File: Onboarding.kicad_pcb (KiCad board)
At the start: 2 copper layers, 45.7 x 45.7 mm, 20 parts, among them J1 Conn_01x02, J2 Conn_01x02, J3 Conn_01x02, J4 Conn_01x02, U2 MC34063A

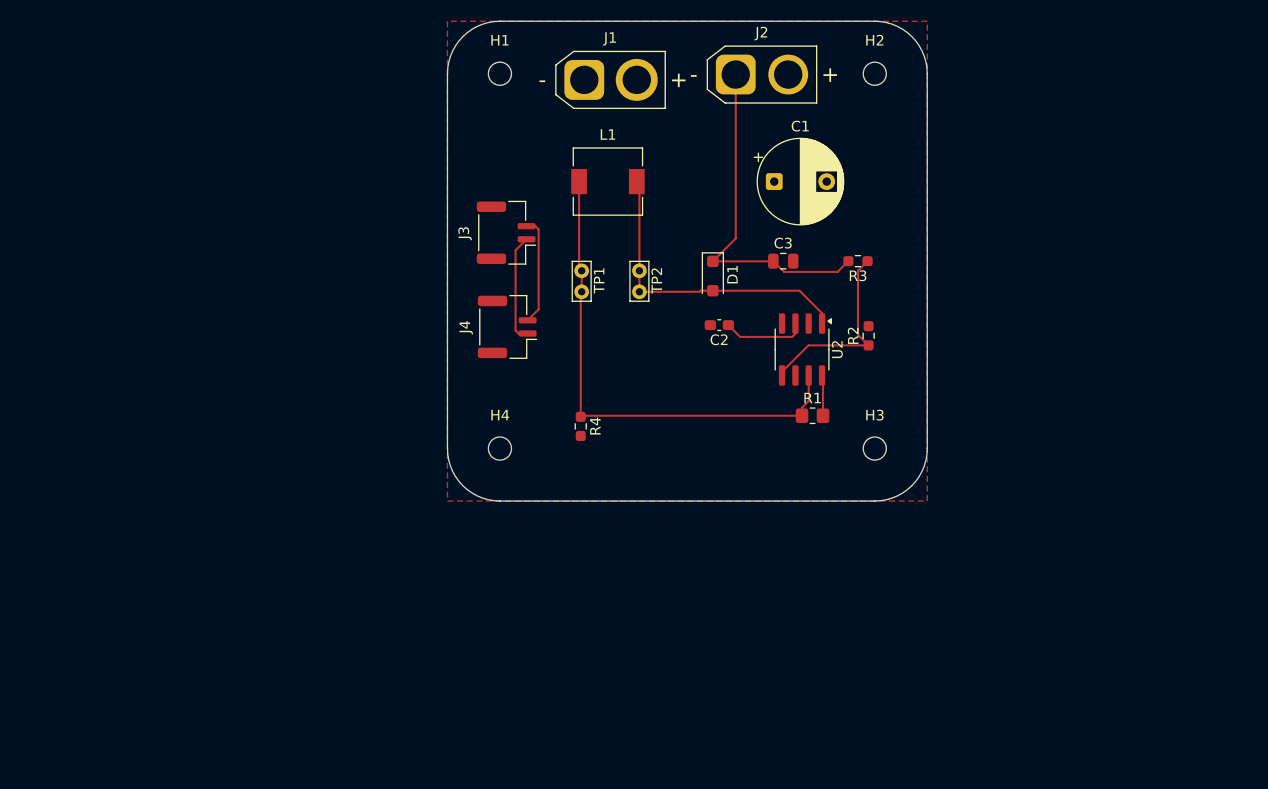
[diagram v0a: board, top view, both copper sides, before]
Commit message: Update PCB
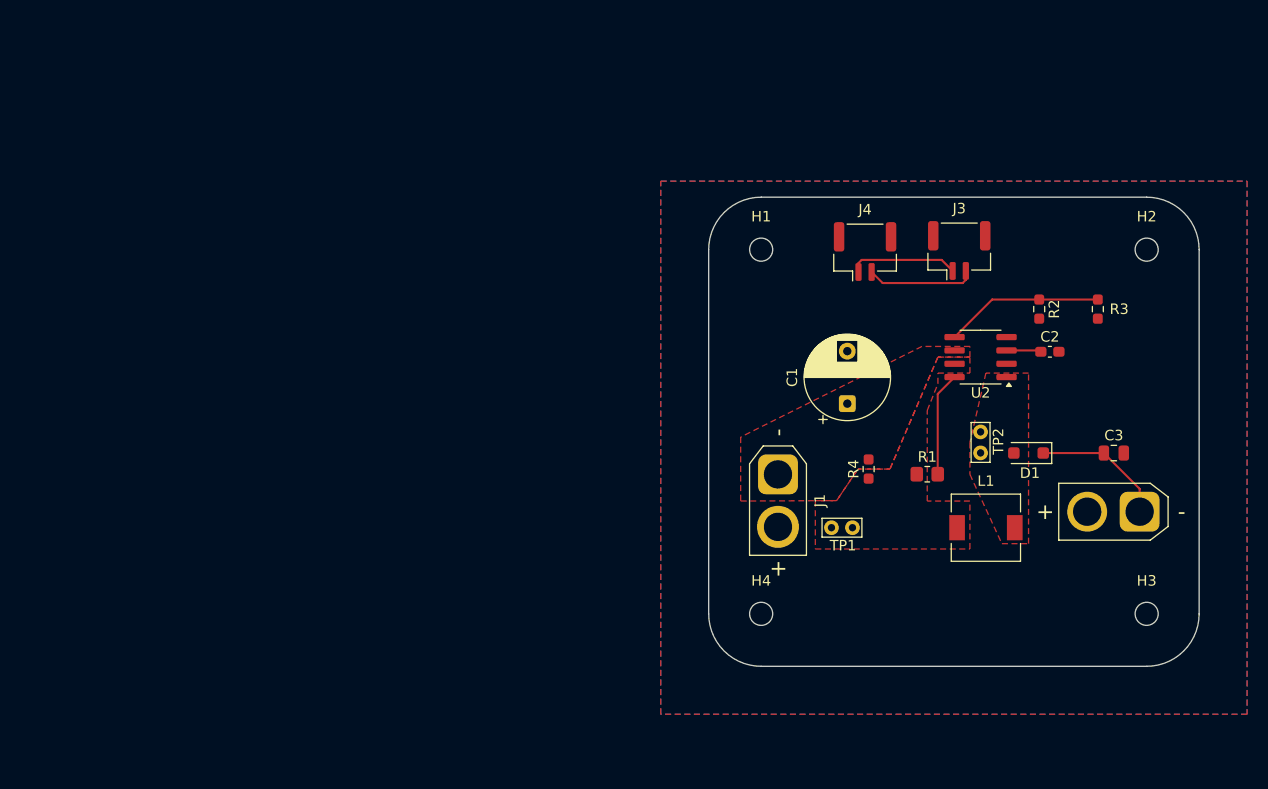
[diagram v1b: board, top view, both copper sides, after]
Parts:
- moved J2 56.7 mm to (253.9, 92.5), turned to 180 degrees
- moved L1 48.8 mm to (239.3, 94.0)
- moved J3 43.2 mm to (236.7, 67.6), turned to 0 degrees
- moved J1 41.9 mm to (219.5, 88.9), turned to -90 degrees
- moved C3 36.4 mm to (251.5, 86.9)
- moved TP2 36.0 mm to (238.8, 86.9)
- moved J4 34.9 mm to (227.8, 67.7), turned to 0 degrees
- moved D1 34.5 mm to (243.3, 86.9), turned to 180 degrees
- moved TP1 32.7 mm to (224.6, 94.0), turned to 0 degrees
- moved C2 31.6 mm to (245.4, 77.2), turned to 0 degrees
- moved H2 30.9 mm to (254.6, 67.5)
- moved H3 30.3 mm to (254.6, 102.2)
- moved H1 30.0 mm to (217.9, 67.5)
- moved H4 29.5 mm to (217.9, 102.2)
- moved R4 27.7 mm to (228.1, 88.4), turned to 90 degrees
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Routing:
- net Net-(U2-I_{PK}): track 47.8 -> 0.00 mm
- net Net-(D1-A): track 29.9 -> 0.00 mm
- net VCC: track 32.5 -> 12.8 mm
- net Net-(U2-DC): track 3.88 -> 9.92 mm
- net Net-(U2-CT): track 7.95 -> 3.32 mm
- net Net-(U2-COMP-): track 18.5 -> 15.1 mm
- added copper zone on B.Cu, net GND
- added copper zone on F.Cu, net GND
- added copper zone on F.Cu, net Net-(D1-A)
- added copper zone on F.Cu, net Net-(U2-I_{PK})
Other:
- board size 45.7 x 45.7 mm -> 46.7 x 44.7 mm

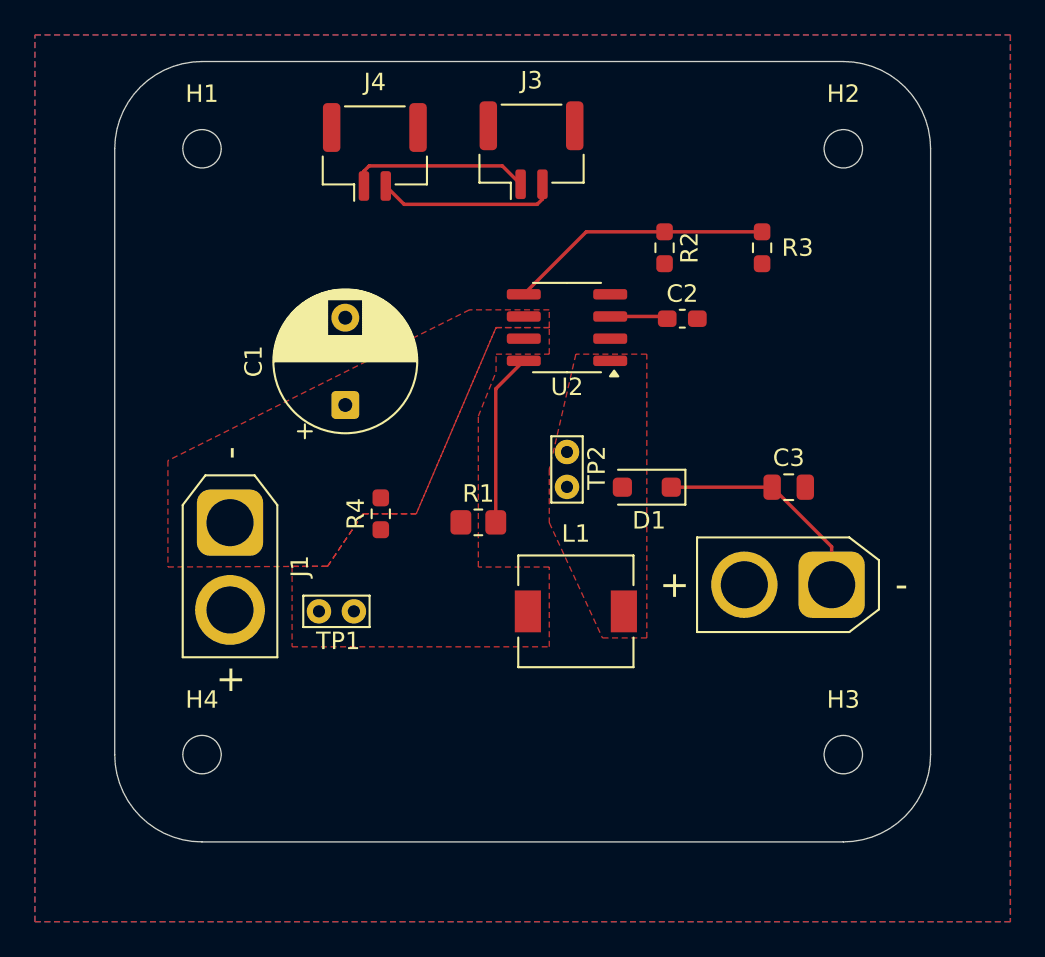
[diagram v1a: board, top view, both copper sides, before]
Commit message: Update Onboarding.kicad_pcb
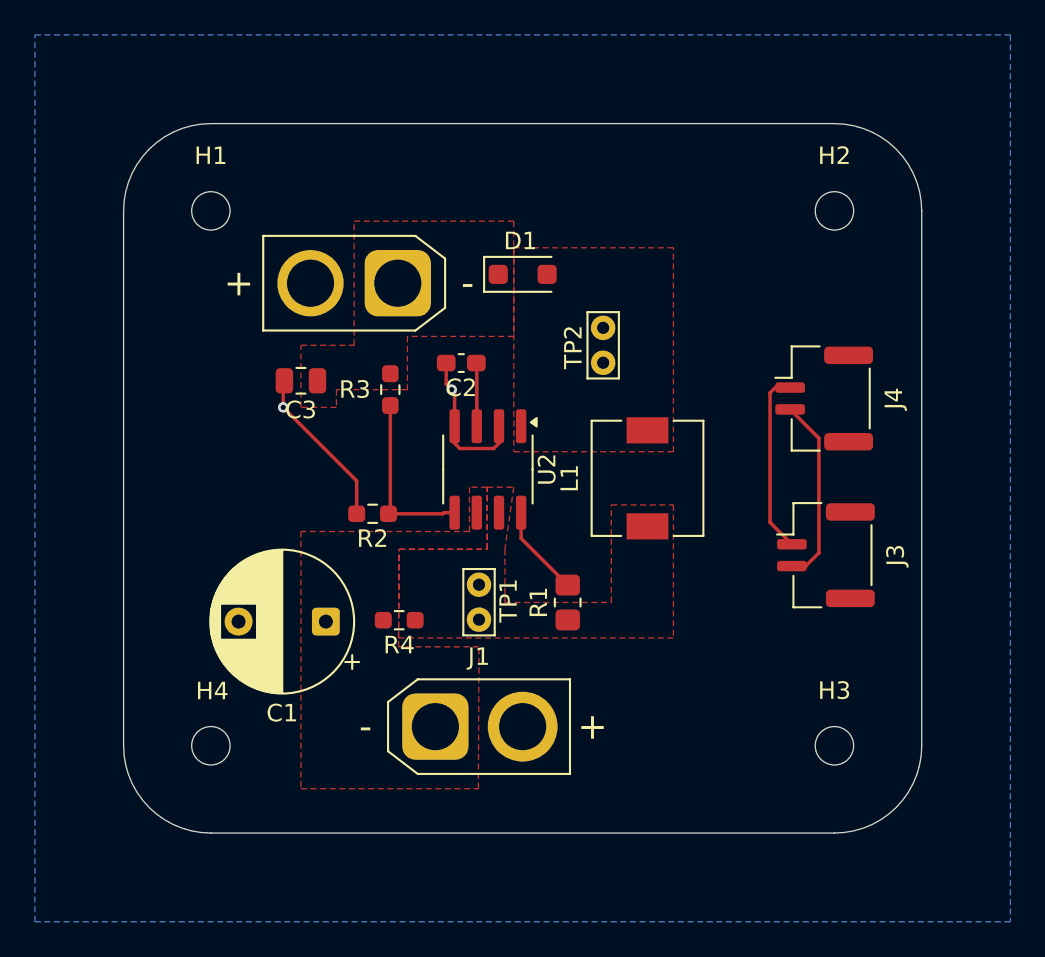
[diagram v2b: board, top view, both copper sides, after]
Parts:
- moved J2 30.3 mm to (229.1, 75.2)
- moved J4 29.4 mm to (253.5, 81.8), turned to -90 degrees
- moved J3 28.7 mm to (253.6, 90.8), turned to -90 degrees
- moved C3 28.6 mm to (223.5, 80.8), turned to 180 degrees
- moved R3 22.8 mm to (228.6, 81.3), turned to 90 degrees
- moved R2 22.6 mm to (227.6, 88.4), turned to 180 degrees
- moved J1 16.6 mm to (231.2, 100.6), turned to 0 degrees
- moved D1 14.1 mm to (236.2, 74.7), turned to 0 degrees
- moved C2 12.9 mm to (232.7, 79.8), turned to 180 degrees
- moved C1 12.5 mm to (224.9, 94.6), turned to 180 degrees
- moved TP2 9.34 mm to (240.8, 77.7), turned to -90 degrees
- moved U2 9.31 mm to (234.2, 85.9), turned to -90 degrees
- moved TP1 9.18 mm to (233.7, 94.5), turned to 90 degrees
- moved L1 8.65 mm to (243.4, 86.4), turned to 90 degrees
- moved R1 6.87 mm to (238.8, 93.5), turned to 90 degrees
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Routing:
- net GND: track 0.00 -> 17.9 mm, vias 0 -> 2
- net VCC: track 12.8 -> 0.00 mm
- net Net-(U2-COMP-): track 15.1 -> 10.1 mm
- net Net-(U2-DC): track 9.92 -> 5.25 mm
- added copper zone on F.Cu, net VCC
- removed copper zone on F.Cu, net GND
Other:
- board size 46.7 x 44.7 mm -> 45.7 x 40.6 mm

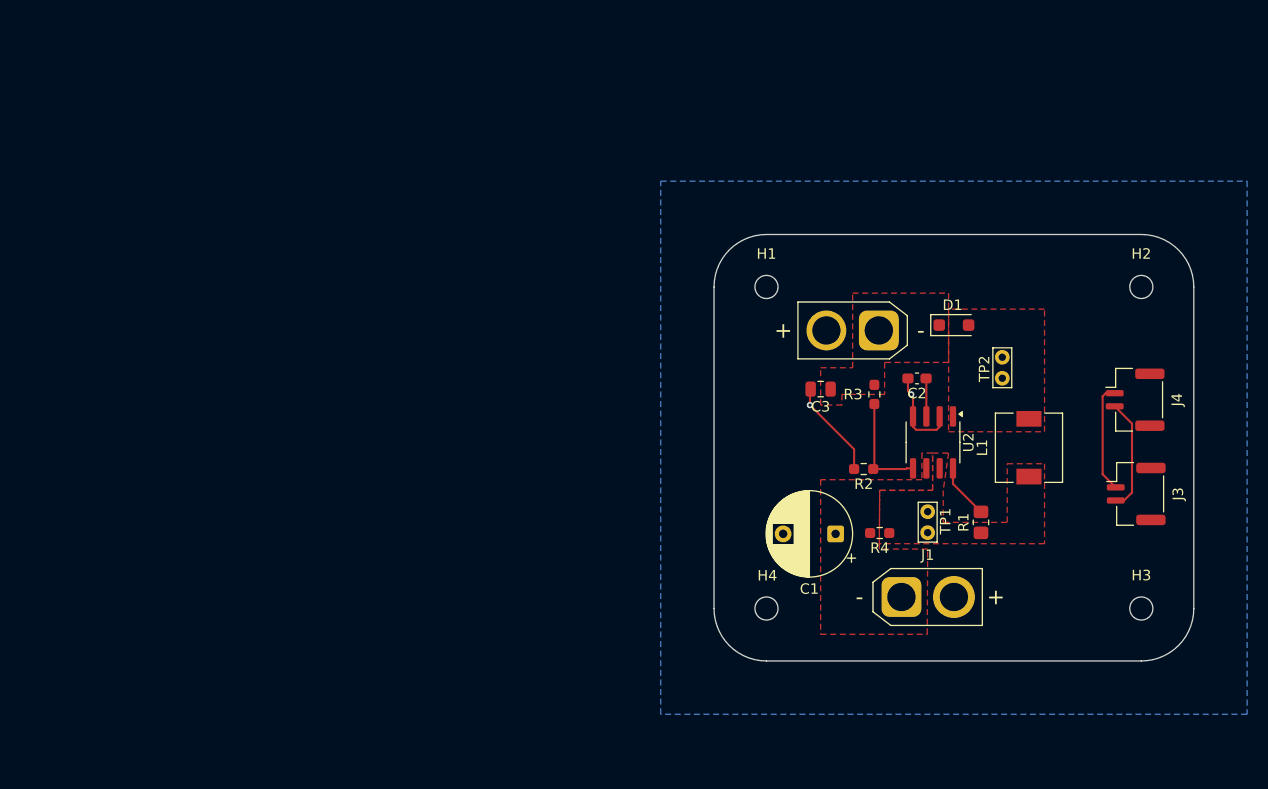
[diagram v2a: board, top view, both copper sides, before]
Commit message: Finish Onboarding
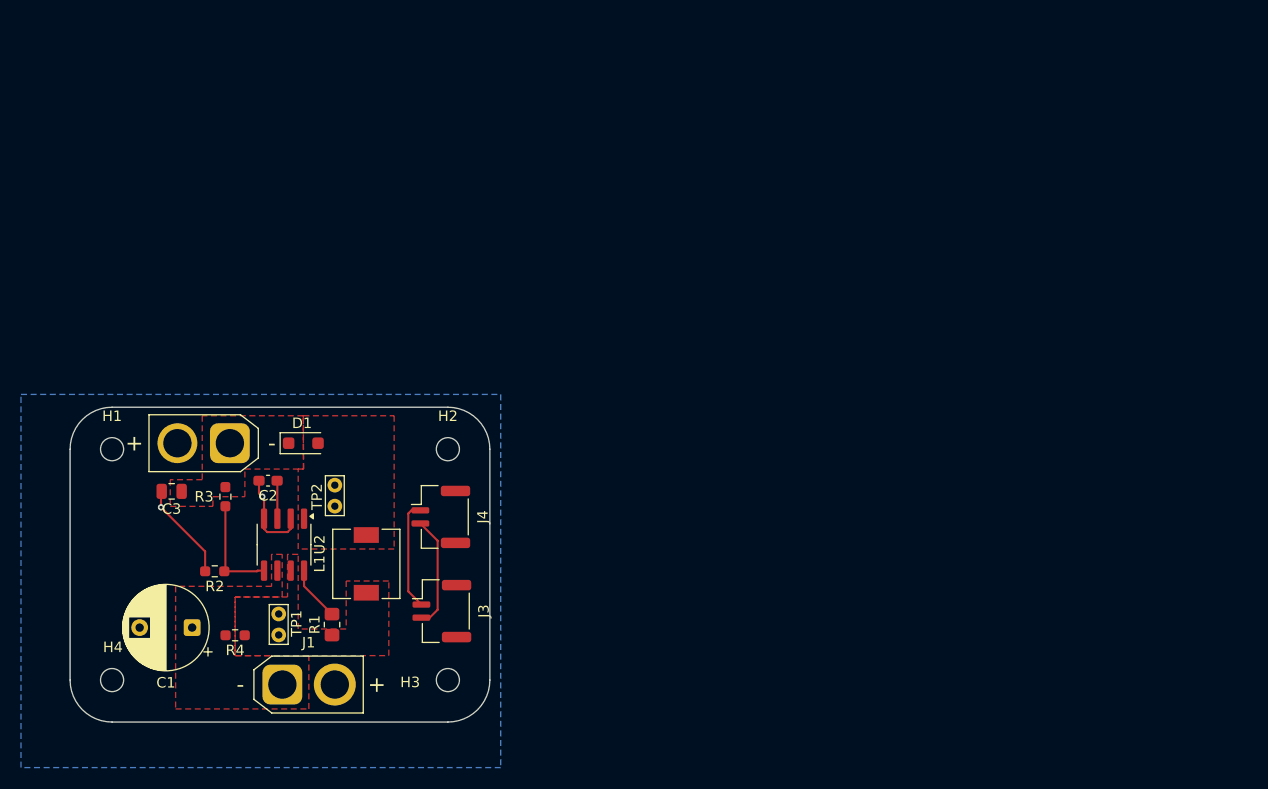
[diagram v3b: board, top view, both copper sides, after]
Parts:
- moved H2 67.9 mm to (188.0, 86.5)
- moved J3 67.1 mm to (187.4, 101.9)
- moved J4 67.1 mm to (187.3, 93.0)
- moved H3 66.4 mm to (188.0, 108.5)
- moved TP2 64.8 mm to (177.2, 89.9)
- moved H1 64.2 mm to (156.0, 86.5)
- moved L1 64.1 mm to (180.2, 97.4)
- moved D1 63.0 mm to (174.2, 85.9)
- moved J2 62.8 mm to (167.2, 85.9)
- moved H4 62.7 mm to (156.0, 108.5)
- moved R1 62.6 mm to (177.0, 103.2)
- moved C2 62.6 mm to (170.9, 89.5)
- moved C3 62.6 mm to (161.7, 90.5)
- moved R2 62.6 mm to (165.8, 98.1)
- moved R3 62.6 mm to (166.8, 91.0)
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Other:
- board size 45.7 x 40.6 mm -> 40 x 30 mm
